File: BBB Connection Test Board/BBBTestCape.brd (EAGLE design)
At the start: 60.9 x 54.3 mm, 27 parts, among them X0 SWTCH_BLCK, X1 SWTCH_BLCK

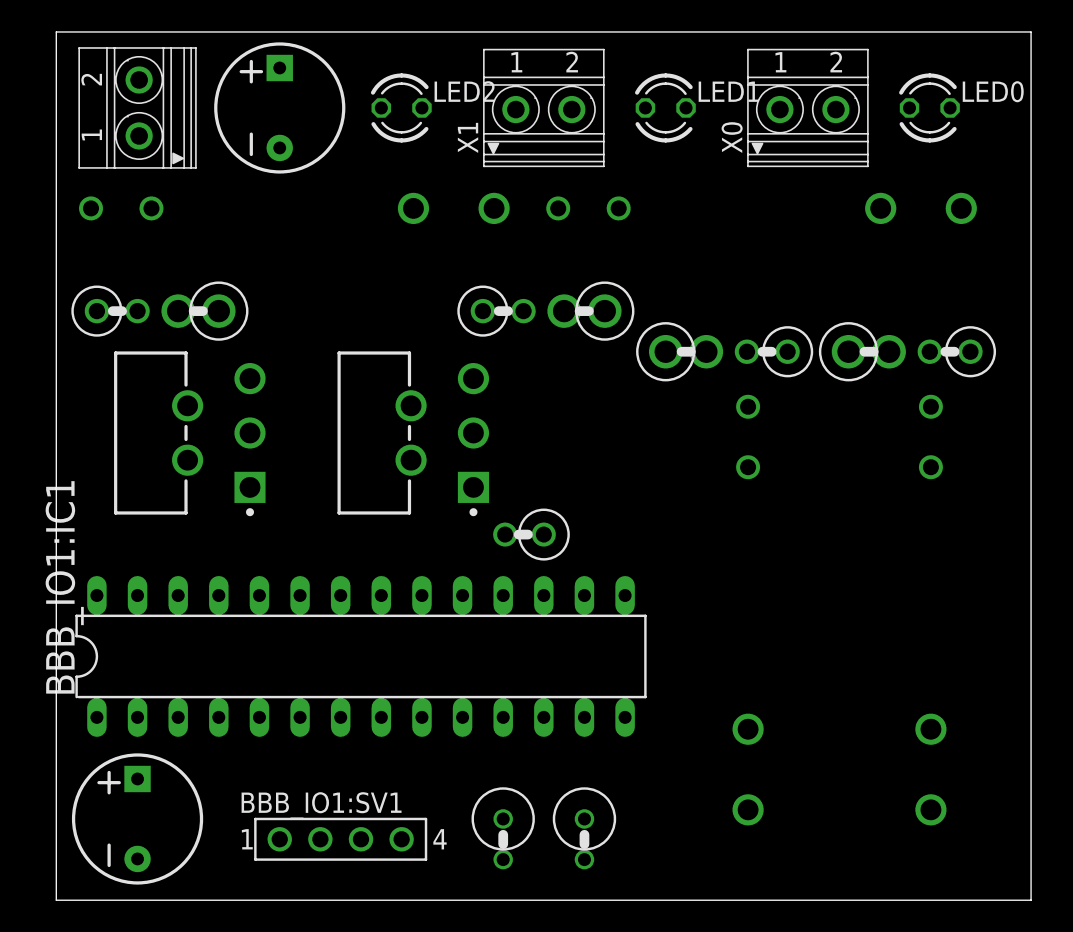
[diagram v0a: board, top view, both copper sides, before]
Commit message: Almost finished with Rev B of connector board. Comestic changes only
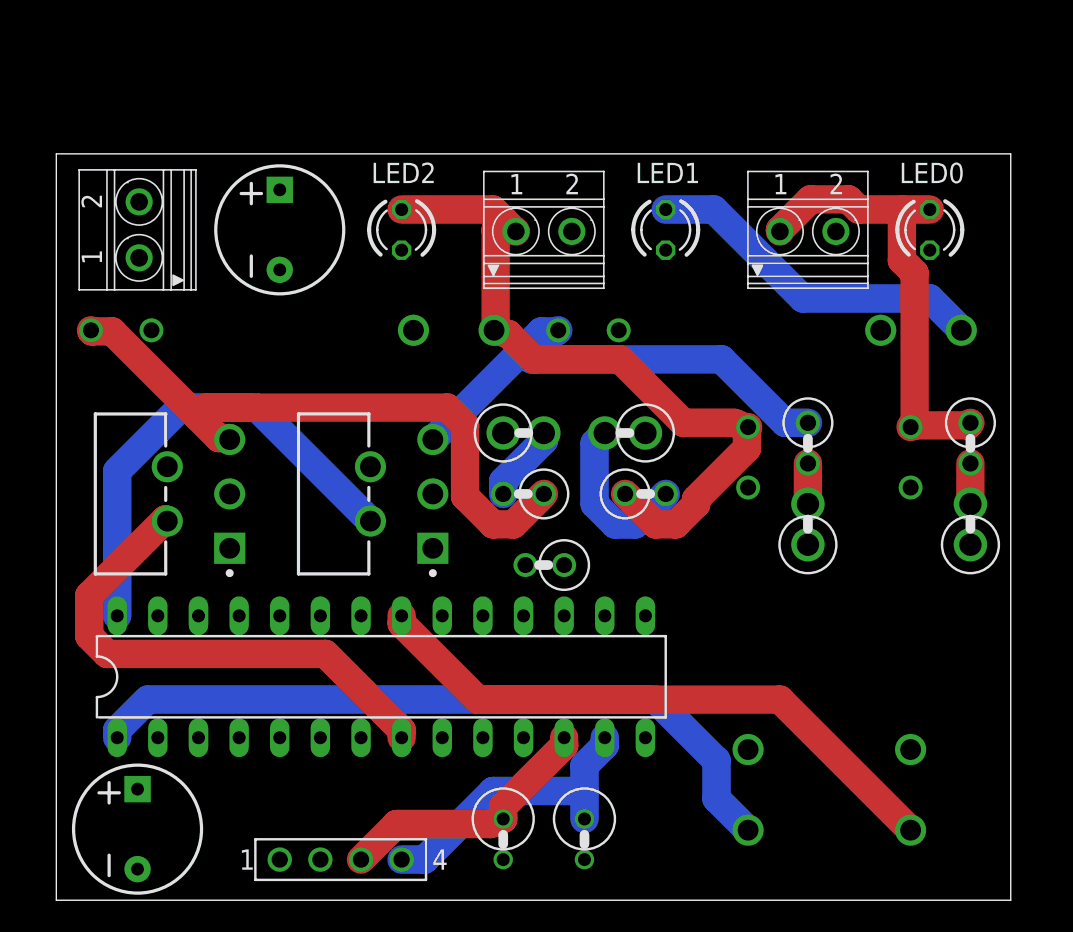
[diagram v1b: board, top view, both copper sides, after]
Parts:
- moved DUAL_12V⇆3V3_1BIT1:3V3_TO_12_1BIT1:D3 27.9 mm to (29.2, 25.4), turned to 180 degrees
- moved DUAL_12V⇆3V3_1BIT1:3V3_TO_12_1BIT1:D4 21.7 mm to (29.2, 29.2), turned to 0 degrees
- moved DUAL_12V⇆3V3_1BIT1:12V_TO_3V3_1BIT1:D5 14.5 mm to (36.8, 25.4)
- moved 3V3_TO_12_1BIT1:D4 13.2 mm to (47.0, 23.5), turned to 90 degrees
- moved 12V_TO_3V3_1BIT1:D6 12.5 mm to (57.1, 23.5), turned to 90 degrees
- moved DUAL_12V⇆3V3_1BIT1:12V_TO_3V3_1BIT1:D6 8.03 mm to (35.6, 29.2)
- moved 12V_PWR_BLK:C1 7.62 mm to (14.0, 41.9)
- moved 12V_PWR_BLK:PWR 7.62 mm to (5.08, 41.9)
- moved 3V3_TO_12_1BIT1:K2 7.62 mm to (58.4, 36.8)
- moved DUAL_12V⇆3V3_1BIT1:3V3_TO_12_1BIT1:K2 7.62 mm to (29.2, 36.8)
- moved LED0 7.62 mm to (54.6, 41.9), turned to 270 degrees
- moved LED1 7.62 mm to (38.1, 41.9), turned to 270 degrees
- moved LED2 7.62 mm to (21.6, 41.9), turned to 270 degrees
- moved X0 7.62 mm to (47.0, 41.9)
- moved X1 7.62 mm to (30.5, 41.9)
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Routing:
- net N$5: track 0.00 -> 45.5 mm
- net N$3: track 0.00 -> 44.9 mm
- net DUAL_12V⇆3V3_1BIT1:3V3_TO_12_1BIT1:N$1: track 0.00 -> 39.8 mm
- net N$7: track 0.00 -> 37.6 mm
- net N$4: track 0.00 -> 31.9 mm
- net 3V3_TO_12_1BIT1:N$1: track 0.00 -> 30.4 mm
- net N$6: track 0.00 -> 29.5 mm
- net N$2: track 0.00 -> 28.2 mm
- net N$1: track 0.00 -> 21.6 mm
- net BBB_IO1:SDA: track 0.00 -> 18.8 mm
- net BBB_IO1:SCL: track 0.00 -> 16.5 mm
- net DUAL_12V⇆3V3_1BIT1:12V_TO_3V3_1BIT1:D$3: track 0.00 -> 10.5 mm
- net DUAL_12V⇆3V3_1BIT1:3V3_TO_12_1BIT1:D$2: track 0.00 -> 4.86 mm
- net 3V3_TO_12_1BIT1:D$2: track 0.00 -> 2.54 mm
- net 12V_TO_3V3_1BIT1:D$3: track 0.00 -> 2.54 mm
- added copper zone on layer 15, net +12V
- added copper zone on layer 15, net +3V3
- added copper zone on layer 2, net GND
- added copper zone on layer 2, net GND3
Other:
- board size 60.9 x 54.3 mm -> 59.7 x 46.7 mm
- board text added: "12V"
- board text added: "3.3V"
- board text added: "GND"
- board text added: "SCL"
- board text added: "SDA"
